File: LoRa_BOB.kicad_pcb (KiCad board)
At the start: 4 copper layers, 23 x 77 mm, 8 parts, among them U1 XC6210B332MR-G, U2 RFM95W-915S2, U3 74HC4050D

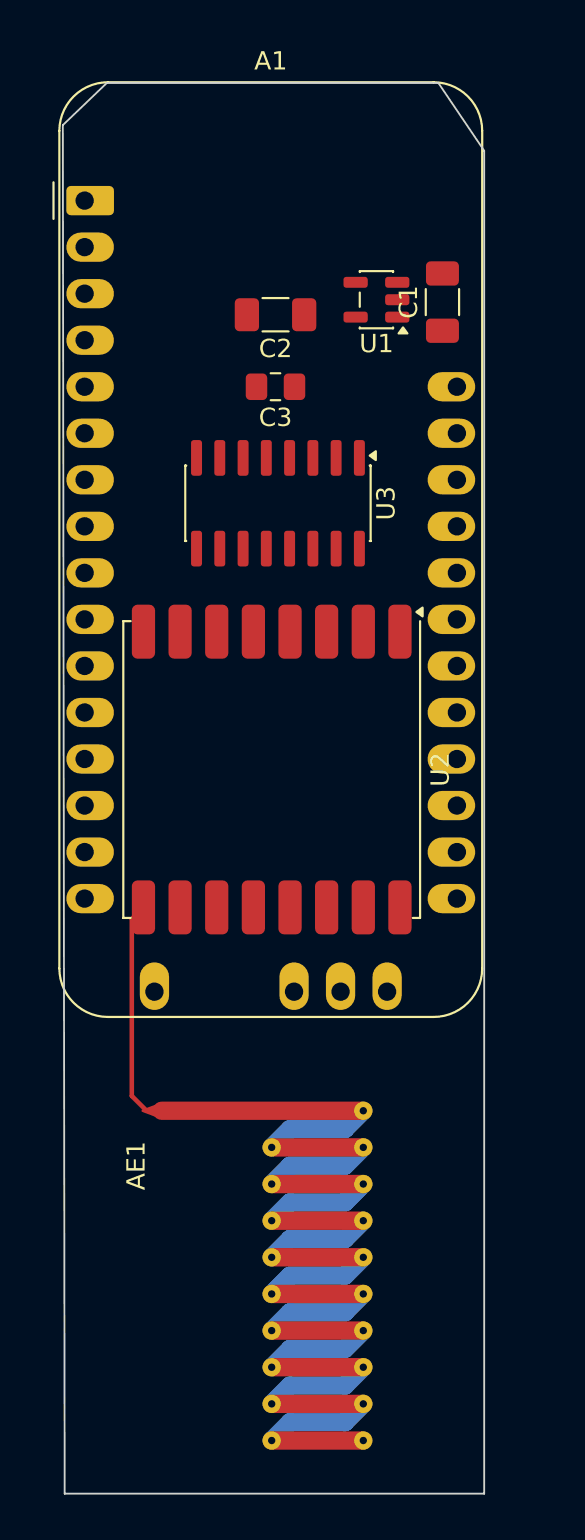
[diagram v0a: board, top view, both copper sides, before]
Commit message: Routed but could be better
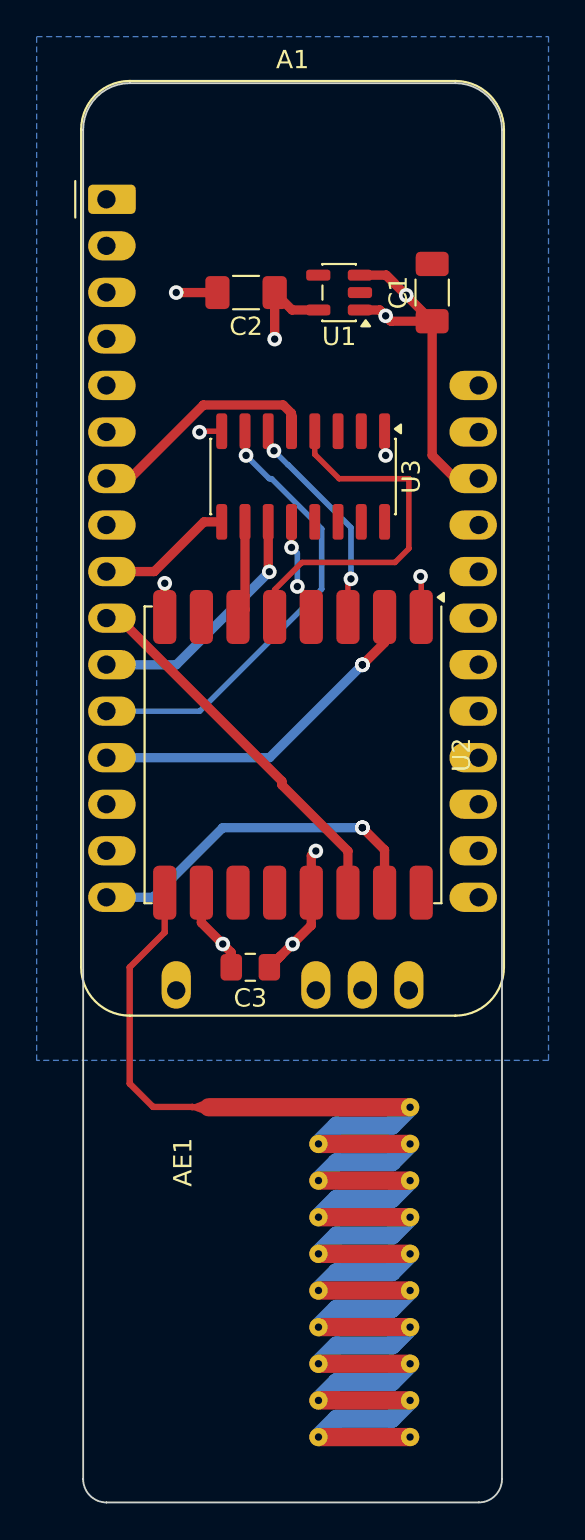
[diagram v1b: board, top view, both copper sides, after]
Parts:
- moved C3 31.7 mm to (254.2, 204.5)
- moved AE1 2.56 mm to (257.2, 221.1)
- moved U1 2.07 mm to (259.1, 167.6)
- moved C2 2.01 mm to (254.0, 167.6)
- moved U3 2.00 mm to (257.1, 177.7)
- moved U2 1.41 mm to (256.6, 192.9)
- moved A1 1.19 mm to (246.4, 162.5)
- moved C1 0.76 mm to (264.2, 167.6)
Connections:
- A1 pad 2: Net-(A1-3V3) -> unconnected-(A1-3V3-Pad2)
- C1 pad 2: Net-(U1-GND) -> GND
- C2 pad 2: Net-(U1-GND) -> GND
- C3 pad 2: Net-(U1-GND) -> GND
- U1 pad 2: Net-(U1-GND) -> GND
- U3 pad 1: Net-(A1-3V3) -> +3V3
- U3 pad 8: unconnected-(U3-GND-Pad8) -> GND
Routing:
- net /MOSI: track 0.00 -> 23.6 mm, vias 0 -> 1
- net Net-(A1-A5): track 0.00 -> 20.8 mm
- net Net-(A1-USB): track 0.00 -> 20.6 mm, vias 0 -> 2
- net /CS_3V: track 0.00 -> 20.5 mm
- net Net-(A1-DIO1): track 0.00 -> 19.6 mm, vias 0 -> 2
- net /MISO: track 0.00 -> 19.2 mm, vias 0 -> 2
- net /SCK: track 0.00 -> 13.7 mm, vias 0 -> 1
- net +3V3: track 0.00 -> 13.6 mm, vias 0 -> 4
- net /CS: track 0.00 -> 12.9 mm
- net GND: track 0.00 -> 12.3 mm, vias 0 -> 5
- net /MOSI_3V: track 0.00 -> 10.9 mm, vias 0 -> 2
- net Net-(A1-A4): track 0.00 -> 7.42 mm
- net /SCK_3V: track 0.00 -> 5.64 mm, vias 0 -> 2
- net Net-(U2-RESET): track 0.00 -> 5.35 mm
- net Net-(AE1-A): track 11.7 -> 15.2 mm
- added copper zone on In2.Cu, net +3V3
- added copper zone on B.Cu, net GND
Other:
- board size 23 x 77 mm -> 22.9 x 77.5 mm
